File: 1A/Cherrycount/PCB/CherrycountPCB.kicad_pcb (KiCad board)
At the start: 2 copper layers, 127 x 91.4 mm, 25 parts, among them J1 Conn_01x02_Female, J2 Conn_01x03_Female, J3 Conn_01x05_Female, J4 Screw_Terminal_01x02, J5 Screw_Terminal_01x02, J6 Screw_Terminal_01x02, Q1 S8550, Q2 S8550

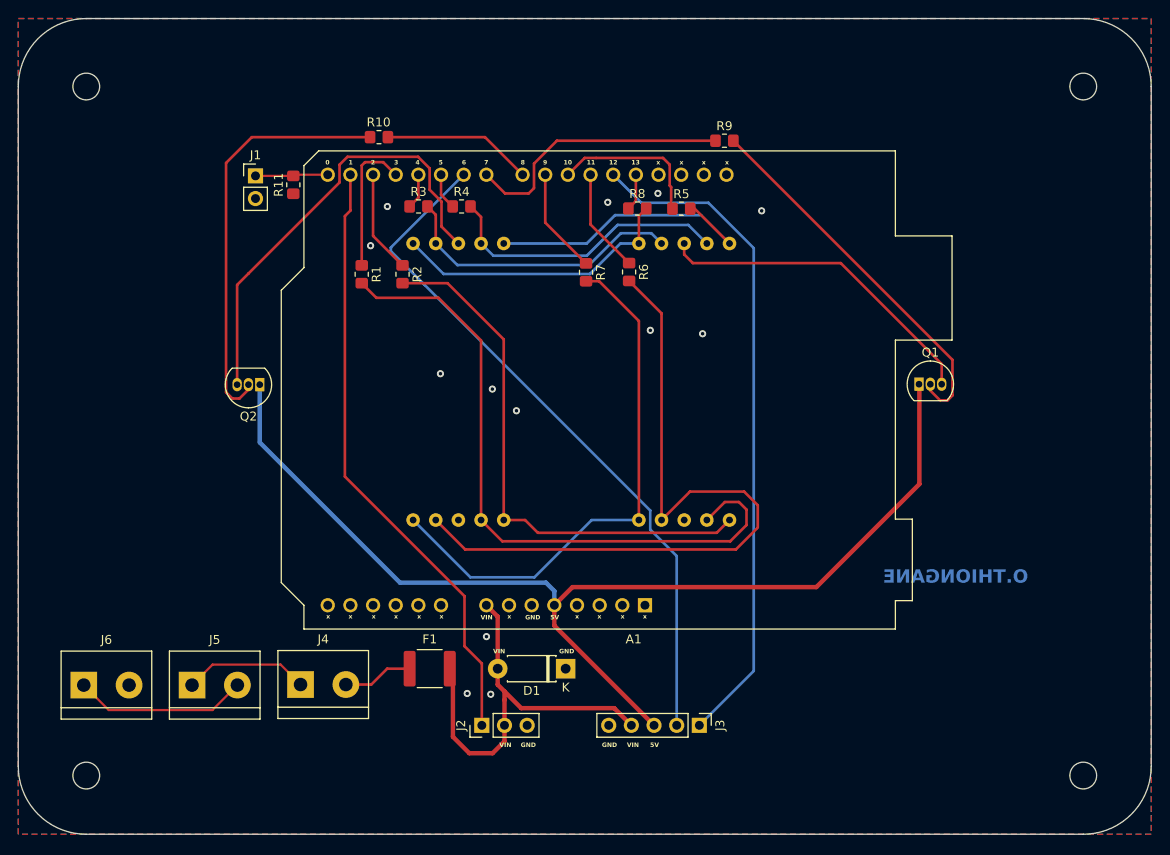
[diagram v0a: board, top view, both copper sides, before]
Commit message: Code final Cherrycount/ajout fichier step ax12
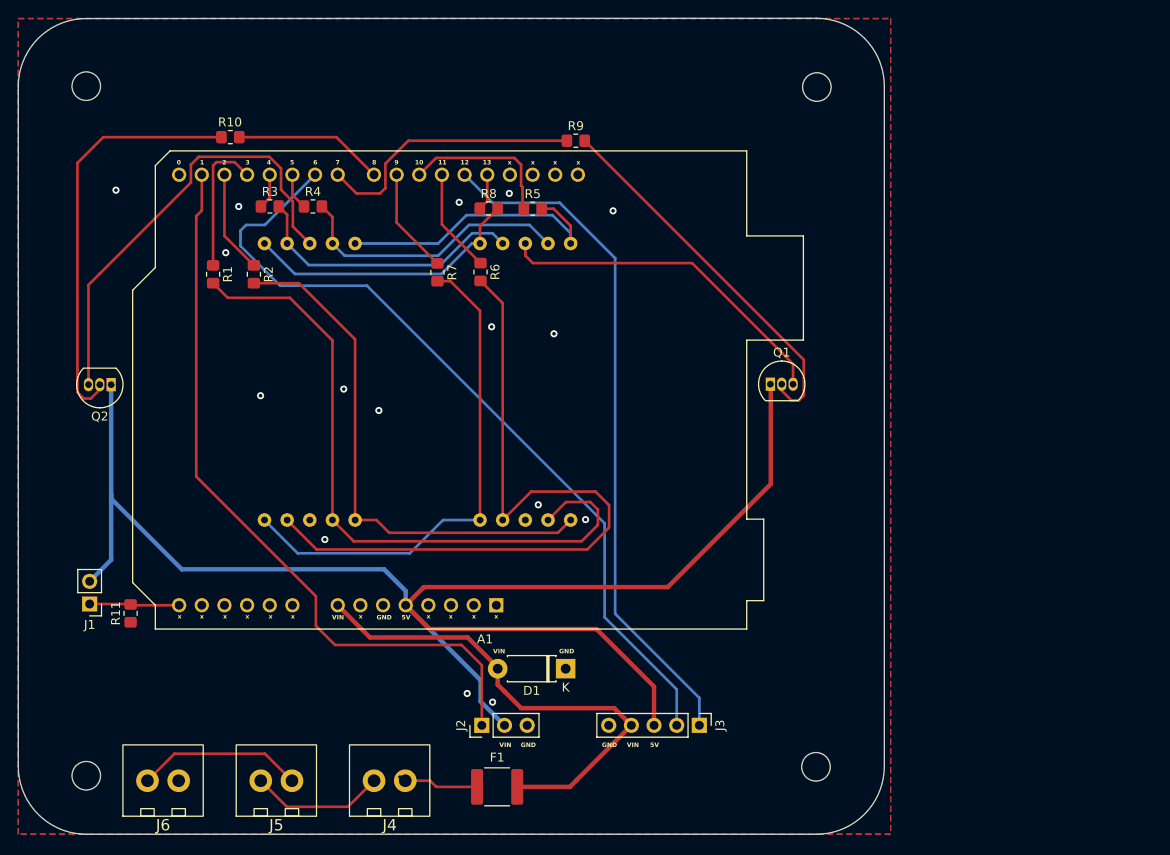
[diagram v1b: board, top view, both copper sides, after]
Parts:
- added REF**: MountingHole_3.2mm_M3, MountingHole:MountingHole_3.2mm_M3, F.Cu at (171.1, 134.0)
- added REF**: MountingHole_3.2mm_M3, MountingHole:MountingHole_3.2mm_M3, F.Cu at (89.3, 57.7)
- added REF**: MountingHole_3.2mm_M3, MountingHole:MountingHole_3.2mm_M3, F.Cu at (171.2, 57.8)
- added REF**: MountingHole_3.2mm_M3, MountingHole:MountingHole_3.2mm_M3, F.Cu at (89.3, 135.0)
- J4, J5, J6: footprint TerminalBlock:TerminalBlock_bornier-2_P5.08mm -> 7seg:180G-2-vertical
- moved J1 51.5 mm to (89.7, 115.8), turned to 180 degrees
- moved R11 51.4 mm to (94.3, 116.8)
- moved G*** 26.8 mm to (163.7, 66.4)
- moved AFF1 17.8 mm to (150.6, 73.8)
- moved R9 16.7 mm to (144.2, 63.8)
- moved AFF2 16.7 mm to (126.4, 73.8)
- moved R1 16.7 mm to (103.5, 78.8)
- moved R3 16.7 mm to (109.9, 71.2)
- moved R4 16.7 mm to (114.7, 71.2)
- moved A1 16.7 mm to (135.3, 115.9)
- moved Q1 16.7 mm to (166.0, 91.1)
- moved Q2 16.7 mm to (92.1, 91.2)
- moved R10 16.7 mm to (105.5, 63.4)
- moved R2 16.7 mm to (108.1, 78.8)
- moved R5 16.7 mm to (139.3, 71.4)
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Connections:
- A1 pad 14: unconnected-(A1-A5-Pad14) -> Net-(A1-A5)
- A1 pad 15: Net-(A1-D0/RX) -> unconnected-(A1-D0/RX-Pad15)
- J1 pad 1: Net-(A1-D0/RX) -> Net-(A1-A5)
- J1 pad 2: GND -> Net-(A1-+5V)
- J2 pad 2: VIN -> Net-(A1-+5V)
- R11 pad 2: Net-(A1-D0/RX) -> Net-(A1-A5)
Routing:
- net Net-(A1-+5V): track 123.8 -> 174.2 mm
- net Conn1x3: track 68.3 -> 83.5 mm
- net D6: track 78.4 -> 92.4 mm
- net Net-(A1-A5): track 0.00 -> 10.1 mm
- net VIN: track 46.8 -> 55.3 mm
- net Net-(A1-D0/RX): track 8.36 -> 0.00 mm
- net Net-(AFF1-g): track 60.7 -> 56.9 mm
- net D12: track 75.2 -> 77.0 mm
- net Net-(J5-Pin_2): track 20.1 -> 18.7 mm
- net Net-(Q1-C): track 37.4 -> 38.7 mm
- net Net-(AFF1-b): track 60.7 -> 59.6 mm
- net Net-(AFF1-c): track 32.8 -> 31.7 mm
- net Net-(AFF1-d): track 32.8 -> 31.7 mm
- net Net-(AFF1-a): track 75.0 -> 76.2 mm
- net Net-(J4-Pin_1): track 14.0 -> 15.1 mm
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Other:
- board size 127 x 91.4 mm -> 97.1 x 91.5 mm
